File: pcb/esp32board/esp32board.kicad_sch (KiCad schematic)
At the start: 88 parts, among them J1 1Wire, J10 NTC5, J11 FuelLevel, J12 12V In, J13 Oil Pressure, J14 Engine, J15 Flywheel, J16 Relays, J2 V2_spare, J5 CAN, J6 NTC1, J7 NTC2, J8 NTC3, J9 NTC4, Q1 BSS138, Q2 BSS138, U1 ESP32-C3-Waveshare, U2 AMS1117-5.0, U3 TJA1050, U4 ADS1115IDGS, U5 ADS1115IDGS, U6 ADS1115IDGS, U7 LM393

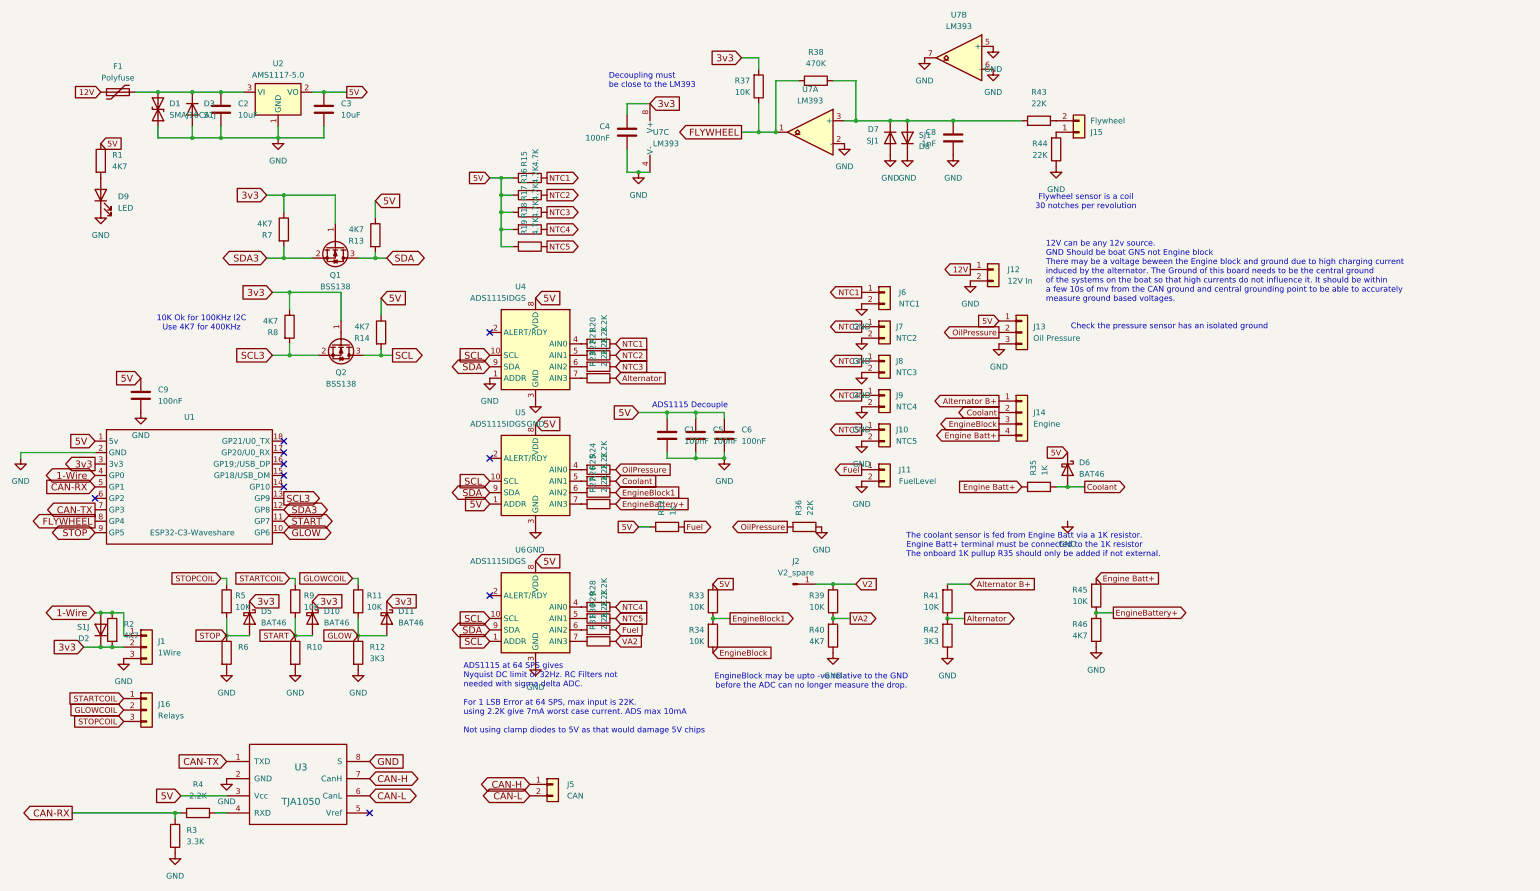
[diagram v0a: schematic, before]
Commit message: Fixed final hardware adjustments
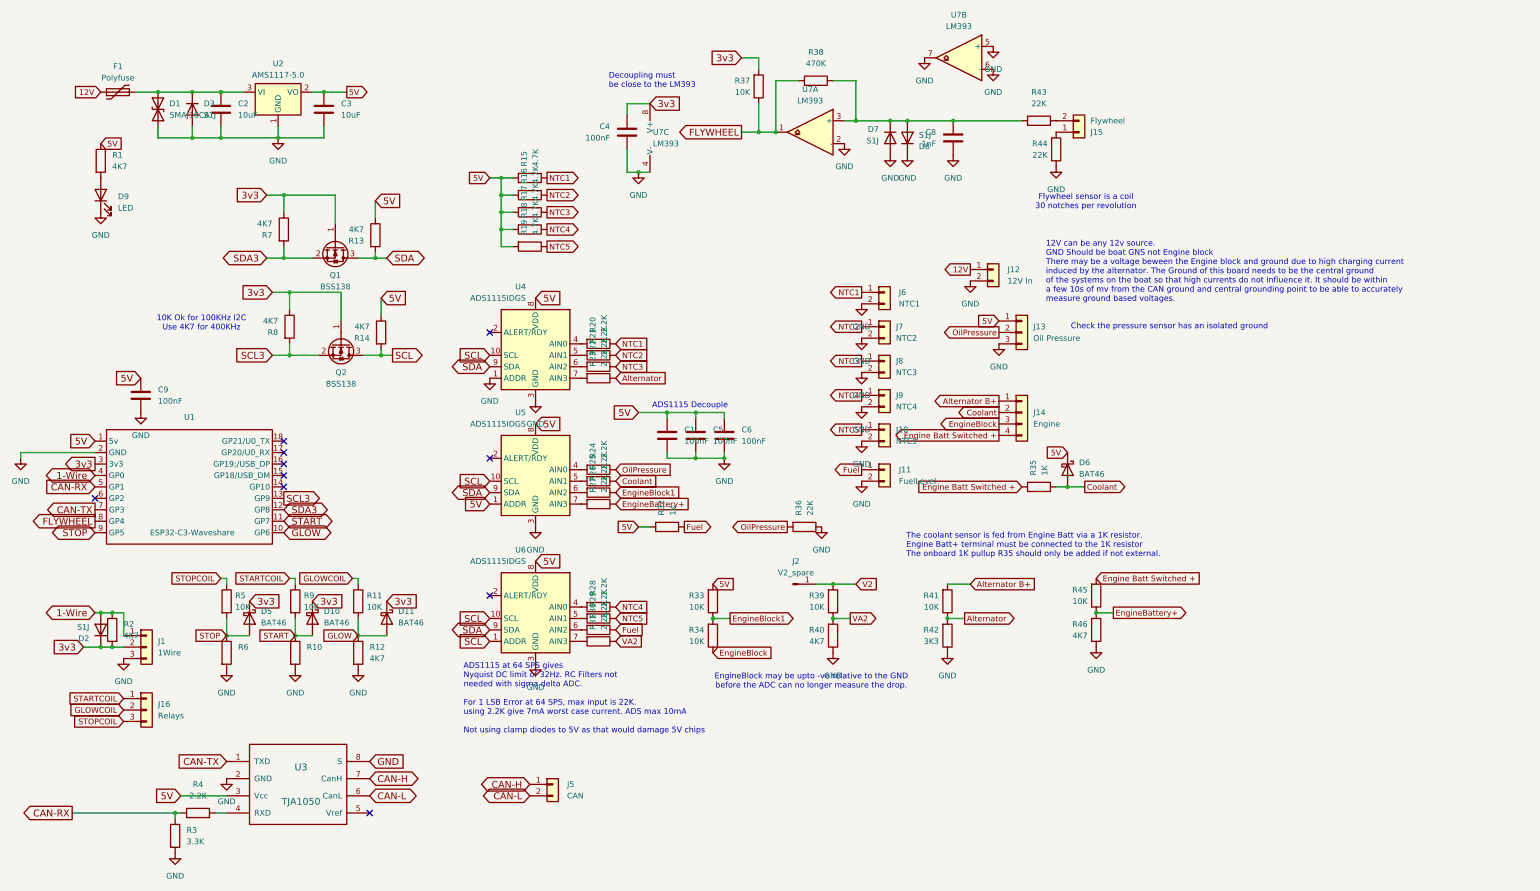
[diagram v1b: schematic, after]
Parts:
- D10, D11, D5, D6: footprint Diode_SMD:Nexperia_CFP3_SOD-123W -> Diode_SMD:D_SOD-123
- D7, D8: value SJ1 -> S1J
- R10, R12, R6: value 3K3 -> 4K7
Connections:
- net Engine Batt+ renamed Engine Batt Switched +
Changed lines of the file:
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@@
 		)
 	)
-	(global_label "Engine Batt+"
+	(global_label "Engine Batt Switched +"
 		(shape input)
-		(at 256.54 137.16 0)
+		(at 240.03 116.84 180)
 		(fields_autoplaced yes)
 		(effects
@@
 				(size 1.27 1.27)
 			)
-			(justify left)
+			(justify right)
 		)
 		(property "Intersheetrefs" "${INTERSHEET_REFS}"
-			(at 272.225 137.16 0)
+			(at 214.0641 116.84 0)
 			(effects
 				(font
 					(size 1.27 1.27)
 				)
-				(justify left)
+				(justify right)
 				(hide yes)
 			)
@@
 		)
 	)
+	(global_label "Engine Batt Switched +"
+		(shape input)
+		(at 256.54 137.16 0)
+		(fields_autoplaced yes)
+		(effects
+			(font
+				(size 1.27 1.27)
+			)
+			(justify left)
+		)
+		(property "Intersheetrefs" "${INTERSHEET_REFS}"
+			(at 282.5059 137.16 0)
+			(effects
+				(font
+					(size 1.27 1.27)
+				)
+				(justify left)
+				(hide yes)
+			)
+		)
+	)
 	(global_label "5V"
 		(shape input)
@@
 		)
 	)
-	(global_label "Engine Batt+"
+	(global_label "Engine Batt Switched +"
 		(shape output)
 		(at 234.95 105.41 180)
@@
 		)
 		(property "Intersheetrefs" "${INTERSHEET_REFS}"
-			(at 219.265 105.41 0)
+			(at 208.9841 105.41 0)
 			(effects
 				(font
@@
 		)
 	)
-	(global_label "Engine Batt+"
-		(shape input)
-		(at 240.03 116.84 180)
-		(fields_autoplaced yes)
-		(effects
-			(font
-				(size 1.27 1.27)
-			)
-			(justify right)
-		)
-		(property "Intersheetrefs" "${INTERSHEET_REFS}"
-			(at 224.345 116.84 0)
-			(effects
-				(font
-					(size 1.27 1.27)
-				)
-				(justify right)
-				(hide yes)
-			)
-		)
-	)
 	(global_label "CAN-L"
 		(shape bidirectional)
@@
 			)
 		)
-		(property "Value" "SJ1"
+		(property "Value" "S1J"
 			(at 217.17 38.735 90)
 			(effects
@@
 			)
 		)
-		(property "Value" "SJ1"
+		(property "Value" "S1J"
 			(at 208.28 40.005 90)
 			(effects
@@
 	)
 	(symbol
-		(lib_name "GND_1")
-		(lib_id "power:GND")
-		(at 250.19 124.46 0)
-		(unit 1)
-		(exclude_from_sim no)
-		(in_bom yes)
-		(on_board yes)
-		(dnp no)
-		(fields_autoplaced yes)
-		(property "Reference" "#PWR039"
-			(at 250.19 130.81 0)
-			(effects
-				(font
-					(size 1.27 1.27)
-				)
-				(hide yes)
-			)
-		)
-		(property "Value" "GND"
-			(at 250.19 129.54 0)
-			(effects
-				(font
-					(size 1.27 1.27)
-				)
-			)
-		)
-		(property "Footprint" ""
-			(at 250.19 124.46 0)
-			(effects
-				(font
-					(size 1.27 1.27)
-				)
-				(hide yes)
-			)
-		)
-		(property "Datasheet" ""
-			(at 250.19 124.46 0)
-			(effects
-				(font
-					(size 1.27 1.27)
-				)
-				(hide yes)
-			)
-		)
-		(property "Description" "Power symbol creates a global label with name \"GND\" , ground"
-			(at 250.19 124.46 0)
-			(effects
-				(font
-					(size 1.27 1.27)
-				)
-				(hide yes)
-			)
-		)
-		(pin "1"
-		)
-		(instances
-			(project "esp32board"
-				(path "/461a08a1-c6de-4673-bbd4-d74d528c254e"
-					(reference "#PWR039")
-					(unit 1)
-				)
-			)
-		)
-	)
-	(symbol
 		(lib_id "Connector_Generic:Conn_01x04")
 		(at 240.03 100.33 0)
@@
 			)
 		)
-		(property "Footprint" "Diode_SMD:Nexperia_CFP3_SOD-123W"
+		(property "Footprint" "Diode_SMD:D_SOD-123"
 			(at 245.745 113.03 0)
 			(effects
@@
 			)
 		)
-		(property "Footprint" "Diode_SMD:Nexperia_CFP3_SOD-123W"
+		(property "Footprint" "Diode_SMD:D_SOD-123"
 			(at 78.105 146.05 0)
 			(effects
@@
 			)
 		)
-		(property "Value" "3K3"
+		(property "Value" "4K7"
 			(at 81.28 154.9399 0)
 			(effects
@@
 			)
 		)
-		(property "Footprint" "Diode_SMD:Nexperia_CFP3_SOD-123W"
+		(property "Footprint" "Diode_SMD:D_SOD-123"
 			(at 94.615 146.05 0)
 			(effects
@@
 			)
 		)
-		(property "Value" "3K3"
+		(property "Value" "4K7"
 			(at 66.04 154.9399 0)
 			(effects
@@
 			)
 		)
-		(property "Value" "3K3"
+		(property "Value" "4K7"
 			(at 95.25 154.9399 0)
 			(effects
@@
 			)
 		)
-		(property "Footprint" "Diode_SMD:Nexperia_CFP3_SOD-123W"
+		(property "Footprint" "Diode_SMD:D_SOD-123"
 			(at 64.135 146.05 0)
 			(effects
